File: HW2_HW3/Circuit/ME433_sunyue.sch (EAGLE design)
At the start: 26 parts

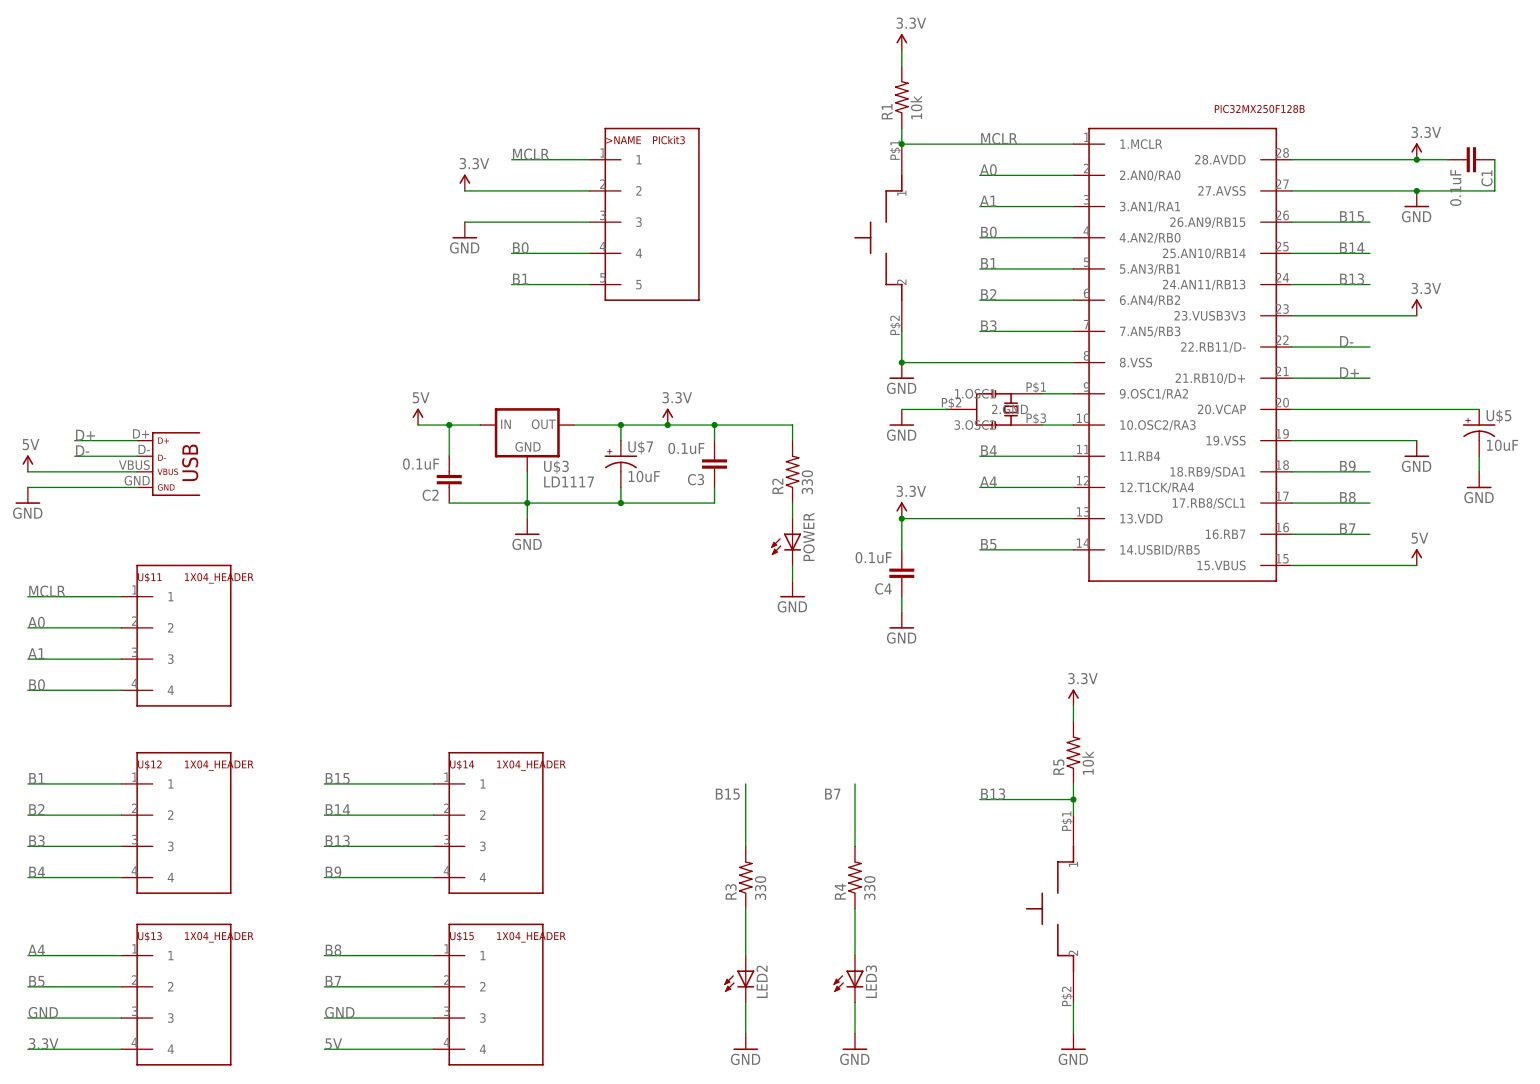
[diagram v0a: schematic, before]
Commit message: HW2_HW3
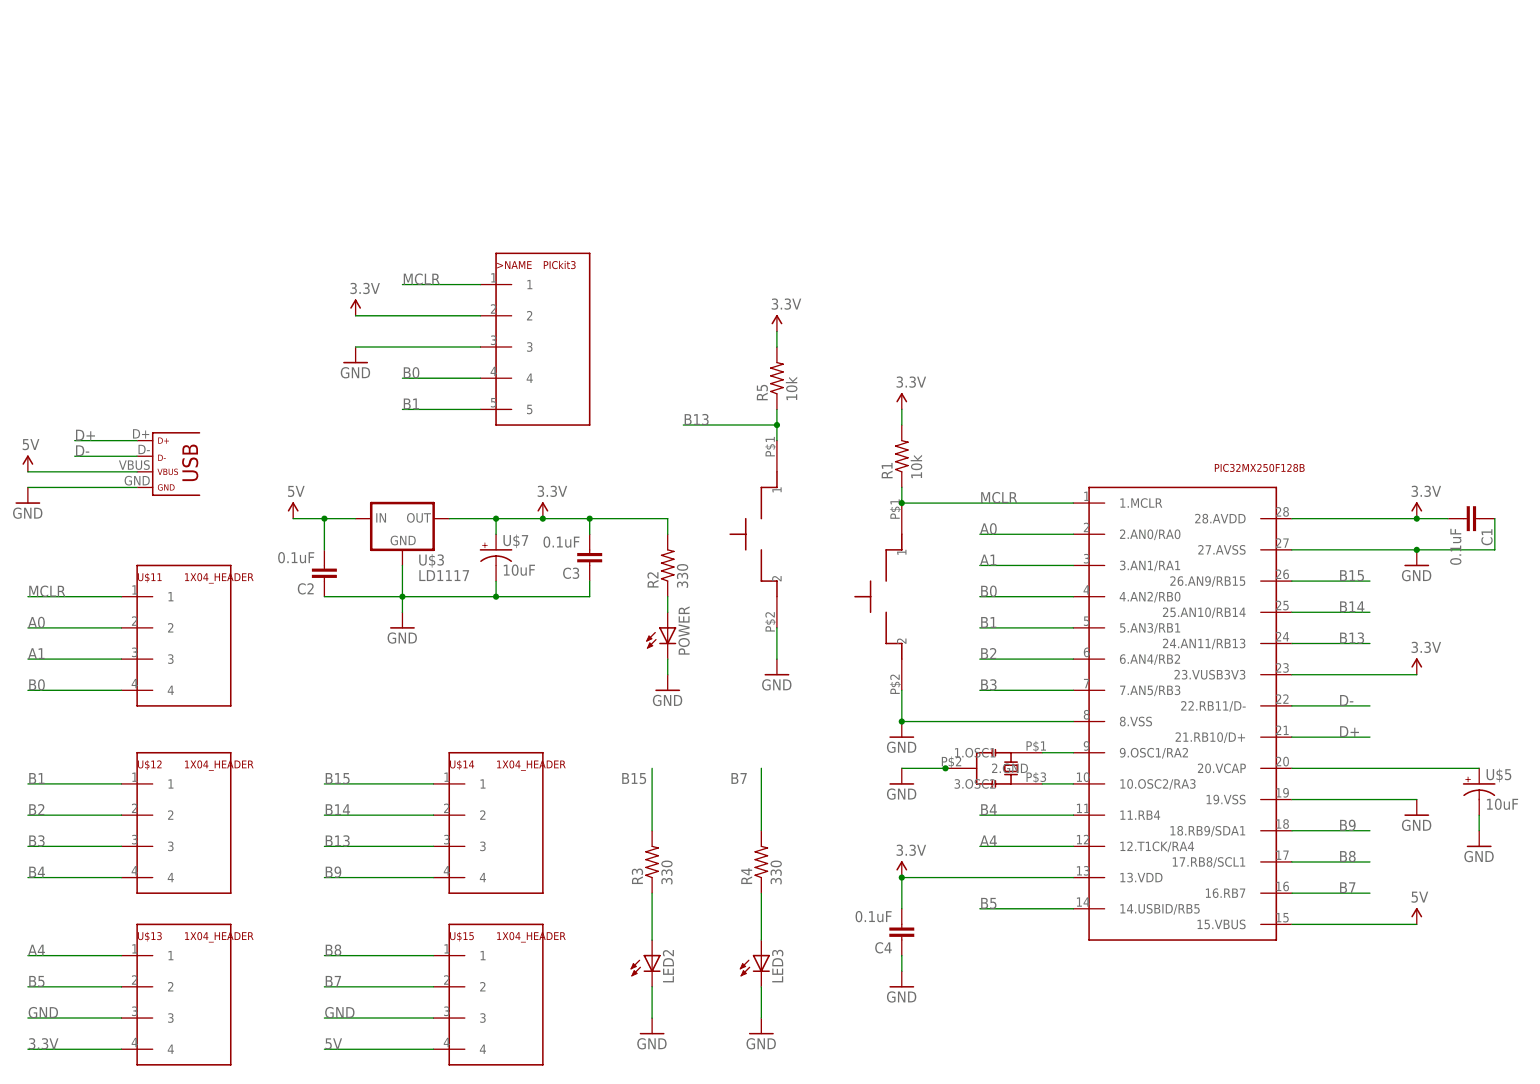
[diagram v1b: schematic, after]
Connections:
- net GND: now also U$2.2.GND
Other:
- moved on the sheet: >NAME, C1, C2, C3, C4, LED2, LED3, POWER, R1, R2, R3, R4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
